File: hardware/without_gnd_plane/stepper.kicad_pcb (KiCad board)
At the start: 6 copper layers, 40 x 40 mm, 130 parts, among them J101 USB-MINI-B-SMD, J102 DRILL, J103 DRILL, J104 DRILL, J105 DRILL, J401 STACK-UP-HIGH, J402 STACK-DOWN, J403 STACK-UP-HIGH, J404 STACK-DOWN, P201 black, P202 green, P301 CON-SENSOR, P302 CON-SENSOR, Q201 AO4438, Q202 AO4421, Q203 2N7002, SW101 Reset, SW102 Erase, U101 AT91SAM3SXB, U102 82400152, U201 TMC2130, U501 LD1117, X101 16Mhz

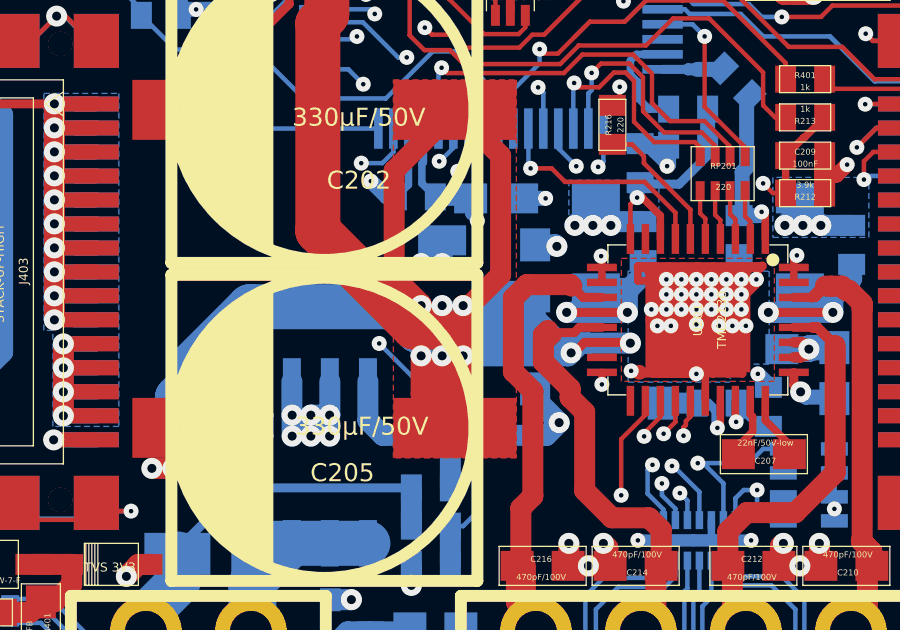
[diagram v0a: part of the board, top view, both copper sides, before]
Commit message: drc check
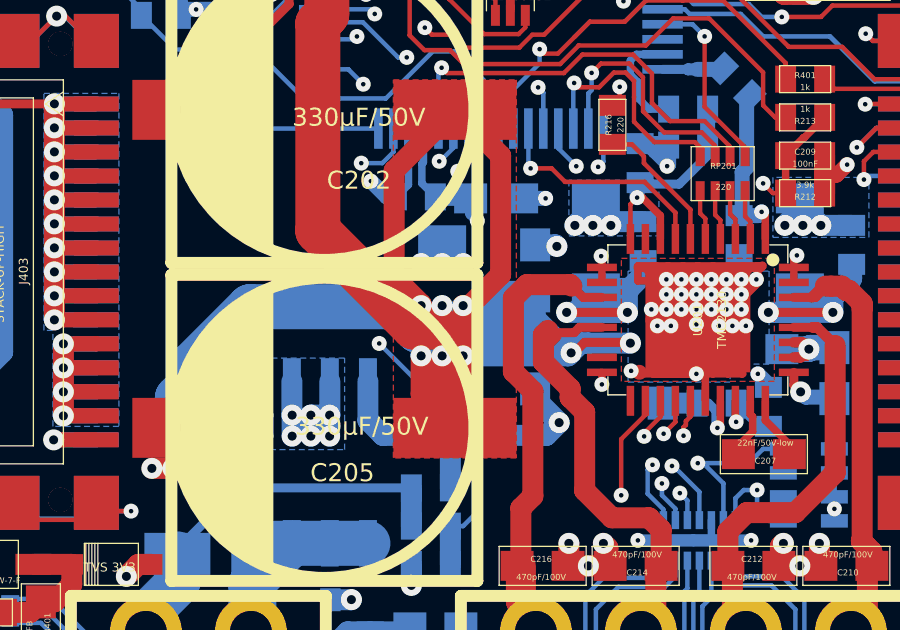
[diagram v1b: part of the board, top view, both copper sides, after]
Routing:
- net 3V3: track 178.7 -> 169.7 mm
- net PWR-ENABLE: track 20.9 -> 19.6 mm
- net STACK-PGND: track 669.1 -> 669.8 mm, vias 141 -> 142
- net BRICKLET-I2C-SCL: track 58.8 -> 58.1 mm
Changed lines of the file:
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@@
     (links 416)
     (no_connects 2)
-    (area 126.671069 72.726549 166.772591 112.825531)
+    (area 125.845139 71.945139 283.420502 165.440043)
     (thickness 1.6002)
     (drawings 63)
-    (tracks 2691)
+    (tracks 2681)
     (zones 0)
     (modules 130)
@@
     (1 GND signal hide)
     (2 IN2.CU signal hide)
-    (3 IN4.CU signal hide)
+    (3 IN4.CU signal)
     (4 VCC signal hide)
-    (31 Rückseite signal)
+    (31 Rückseite signal hide)
     (32 B.Adhes user)
     (33 F.Adhes user)
@@
   )
   (setup
-    (last_trace_width 0.50038)
+    (last_trace_width 0.1524)
     (user_trace_width 0.1524)
     (user_trace_width 0.25)
@@
     (aux_axis_origin 126.725 72.775)
     (grid_origin 126.725 72.775)
-    (visible_elements FFFFBFFF)
+    (visible_elements FFFF3FFF)
     (pcbplotparams
-      (layerselection 0x010fc_80000007)
+      (layerselection 0x00000_00000008)
       (usegerberextensions true)
       (excludeedgelayer true)
@@
   (segment (start 160.1912 94.487) (end 161.6493 94.487) (width 0.1498) (layer Vorderseite) (net 1))
   (segment (start 160.1019 94.3977) (end 160.1912 94.487) (width 0.1498) (layer Vorderseite) (net 1))
-  (segment (start 160.7222 94.487) (end 161.6493 94.487) (width 0.1498) (layer IN4.CU) (net 1))
-  (segment (start 161.6493 94.487) (end 162.1652 93.9711) (width 0.1498) (layer IN4.CU) (net 1))
-  (segment (start 160.7222 97.8778) (end 157.9 100.7) (width 0.148) (layer IN4.CU) (net 1))
-  (segment (start 160.7222 94.487) (end 160.7222 97.8778) (width 0.1498) (layer IN4.CU) (net 1))
   (via (at 162.1652 93.8151) (size 0.5) (layers Vorderseite Rückseite) (net 1))
   (segment (start 162.1652 93.9711) (end 162.1652 93.8151) (width 0.1498) (layer IN4.CU) (net 1))
@@
   (segment (start 165.6 82.6) (end 165.6 82.9493) (width 0.701) (layer Rückseite) (net 1))
   (segment (start 164.7 81.7) (end 165.6 82.6) (width 0.701) (layer Rückseite) (net 1))
+  (segment (start 155.3247 100.0712) (end 155.3247 100.0753) (width 0.1524) (layer IN4.CU) (net 2))
+  (segment (start 154.2529 101.1471) (end 148.2122 101.1471) (width 0.1524) (layer IN4.CU) (net 2))
+  (segment (start 155.3247 100.0753) (end 154.2529 101.1471) (width 0.1524) (layer IN4.CU) (net 2))
   (segment (start 150.875 89.8) (end 152.8 87.875) (width 0.1524) (layer IN4.CU) (net 2))
   (segment (start 157.825 88.05) (end 157.825 89.9025) (width 0.1524) (layer IN4.CU) (net 2))
@@
   (segment (start 129.275 103.05) (end 129.275 102.6888) (width 0.1498) (layer Rückseite) (net 2))
   (segment (start 129.275 102.6888) (end 129.6435 102.3203) (width 0.1498) (layer Rückseite) (net 2))
-  (segment (start 155.3247 100.0712) (end 154.8772 99.6237) (width 0.1498) (layer IN4.CU) (net 2))
-  (segment (start 154.8772 99.6237) (end 153.8699 99.6237) (width 0.1498) (layer IN4.CU) (net 2))
-  (segment (start 153.8699 99.6237) (end 153.676 99.8176) (width 0.1498) (layer IN4.CU) (net 2))
-  (segment (start 153.676 99.8176) (end 153.676 100.3613) (width 0.1498) (layer IN4.CU) (net 2))
-  (segment (start 153.676 100.3613) (end 152.8902 101.1471) (width 0.1498) (layer IN4.CU) (net 2))
-  (segment (start 152.8902 101.1471) (end 148.2122 101.1471) (width 0.1498) (layer IN4.CU) (net 2))
   (segment (start 148.2122 101.1471) (end 147.0391 102.3202) (width 0.1498) (layer IN4.CU) (net 2))
   (segment (start 147.0391 102.3202) (end 129.6435 102.3202) (width 0.1498) (layer IN4.CU) (net 2))
@@
   (segment (start 147.69968 88.02262) (end 147.69968 89.27468) (width 0.148) (layer Rückseite) (net 13))
   (segment (start 147.69968 89.27468) (end 147.775 89.35) (width 0.148) (layer Rückseite) (net 13))
-  (segment (start 145.9965 88.6535) (end 148 86.65) (width 0.1524) (layer IN4.CU) (net 14))
+  (segment (start 146.4144 95.9356) (end 146.4144 91.7856) (width 0.1524) (layer IN4.CU) (net 14))
+  (segment (start 146.725 87.95) (end 148.025 86.65) (width 0.1524) (layer IN4.CU) (net 14))
+  (segment (start 146.725 91.475) (end 146.725 87.95) (width 0.1524) (layer IN4.CU) (net 14))
+  (segment (start 146.4144 91.7856) (end 146.725 91.475) (width 0.1524) (layer IN4.CU) (net 14))
   (segment (start 148.19752 86.82252) (end 148.025 86.65) (width 0.1524) (layer Rückseite) (net 14))
-  (via (at 148.025 86.65) (size 0.5) (drill 0.15) (layers Vorderseite Rückseite) (net 14))
   (segment (start 148.19752 86.82252) (end 148.19752 88.02262) (width 0.1524) (layer Rückseite) (net 14))
-  (segment (start 148 86.65) (end 148.025 86.65) (width 0.1524) (layer IN4.CU) (net 14))
+  (via (at 148.025 86.65) (size 0.5) (drill 0.15) (layers Vorderseite Rückseite) (net 14))
   (segment (start 151.8204 97.8074) (end 152.2084 98.1954) (width 0.1498) (layer IN4.CU) (net 14))
   (segment (start 151.1827 97.8074) (end 151.8204 97.8074) (width 0.1498) (layer IN4.CU) (net 14))
@@
   (segment (start 148.9632 97.25) (end 149.7593 98.0461) (width 0.1498) (layer IN4.CU) (net 14))
   (segment (start 147.7288 97.25) (end 148.9632 97.25) (width 0.1498) (layer IN4.CU) (net 14))
-  (segment (start 146.3999 95.9211) (end 147.7288 97.25) (width 0.1498) (layer IN4.CU) (net 14))
-  (segment (start 146.3999 93.8433) (end 146.3999 95.9211) (width 0.1498) (layer IN4.CU) (net 14))
-  (segment (start 145.4024 92.8458) (end 146.3999 93.8433) (width 0.1498) (layer IN4.CU) (net 14))
-  (segment (start 145.4024 92.2892) (end 145.4024 92.8458) (width 0.1498) (layer IN4.CU) (net 14))
-  (segment (start 144.9014 91.7882) (end 145.4024 92.2892) (width 0.1498) (layer IN4.CU) (net 14))
-  (segment (start 144.9014 90.5624) (end 144.9014 91.7882) (width 0.1498) (layer IN4.CU) (net 14))
-  (segment (start 145.9965 89.4673) (end 144.9014 90.5624) (width 0.1498) (layer IN4.CU) (net 14))
+  (segment (start 146.4144 95.9356) (end 147.7288 97.25) (width 0.1498) (layer IN4.CU) (net 14))
   (segment (start 152.6007 97.8031) (end 152.2084 98.1954) (width 0.1498) (layer Vorderseite) (net 14))
   (segment (start 152.6007 97.0975) (end 152.6007 97.8031) (width 0.1498) (layer Vorderseite) (net 14))
   (via (at 152.2084 98.1954) (size 0.5) (layers Vorderseite Rückseite) (net 14))
-  (segment (start 145.9965 88.6535) (end 145.9965 89.4673) (width 0.148) (layer IN4.CU) (net 14))
   (segment (start 150.7447 87.0053) (end 150.7447 86.6323) (width 0.1524) (layer Vorderseite) (net 15))
   (via (at 150.7447 86.6323) (size 0.5) (layers Vorderseite Rückseite) (net 15))
@@
   (segment (start 164.0182 94.3977) (end 165.8981 94.3977) (width 0.1498) (layer Rückseite) (net 22))
   (segment (start 163.9963 94.3758) (end 164.0182 94.3977) (width 0.1498) (layer Rückseite) (net 22))
+  (segment (start 144.825 92.525) (end 145.525 92.525) (width 0.70104) (layer Rückseite) (net 23))
+  (via (at 145.525 92.525) (size 0.7) (drill 0.3) (layers Vorderseite Rückseite) (net 23))
   (segment (start 157.325 81.175) (end 156.82452 81.175) (width 0.70104) (layer Vorderseite) (net 23))
   (segment (start 156.82452 81.175) (end 155.92452 80.275) (width 0.70104) (layer Vorderseite) (net 23))
@@
     (polygon
       (pts
-        (xy 149.05 89.75) (xy 149.05 91.45) (xy 152.05 91.45) (xy 152.05 89.75)
+        (xy 149.05 89.75) (xy 149.05 91.6) (xy 152.05 91.6) (xy 152.05 89.75)
       )
     )
@@
       )
     )
+  )
+  (zone (net 23) (net_name STACK-PGND) (layer Rückseite) (hatch edge 0.508)
+    (connect_pads yes (clearance 0.15))
+    (min_thickness 0.3)
+    (fill yes (arc_segments 16) (thermal_gap 0.3) (thermal_bridge_width 0.3))
+    (polygon
+      (pts
+        (xy 138.125 95.675) (xy 138.125 98.725) (xy 141.575 98.725) (xy 141.575 95.675)
+      )
+    )
